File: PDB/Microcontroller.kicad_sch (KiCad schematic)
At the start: 14 parts, among them J4 Conn_01x02_Pin, U10 Thermal Resistor, U2 ESP32-DEVKIT-C, U6 TJA1050T/CM,118, U7 SparkFun: ISM330DHCX, MMC5983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, U8 SDIO Card Breakout Board, U9 AM2302

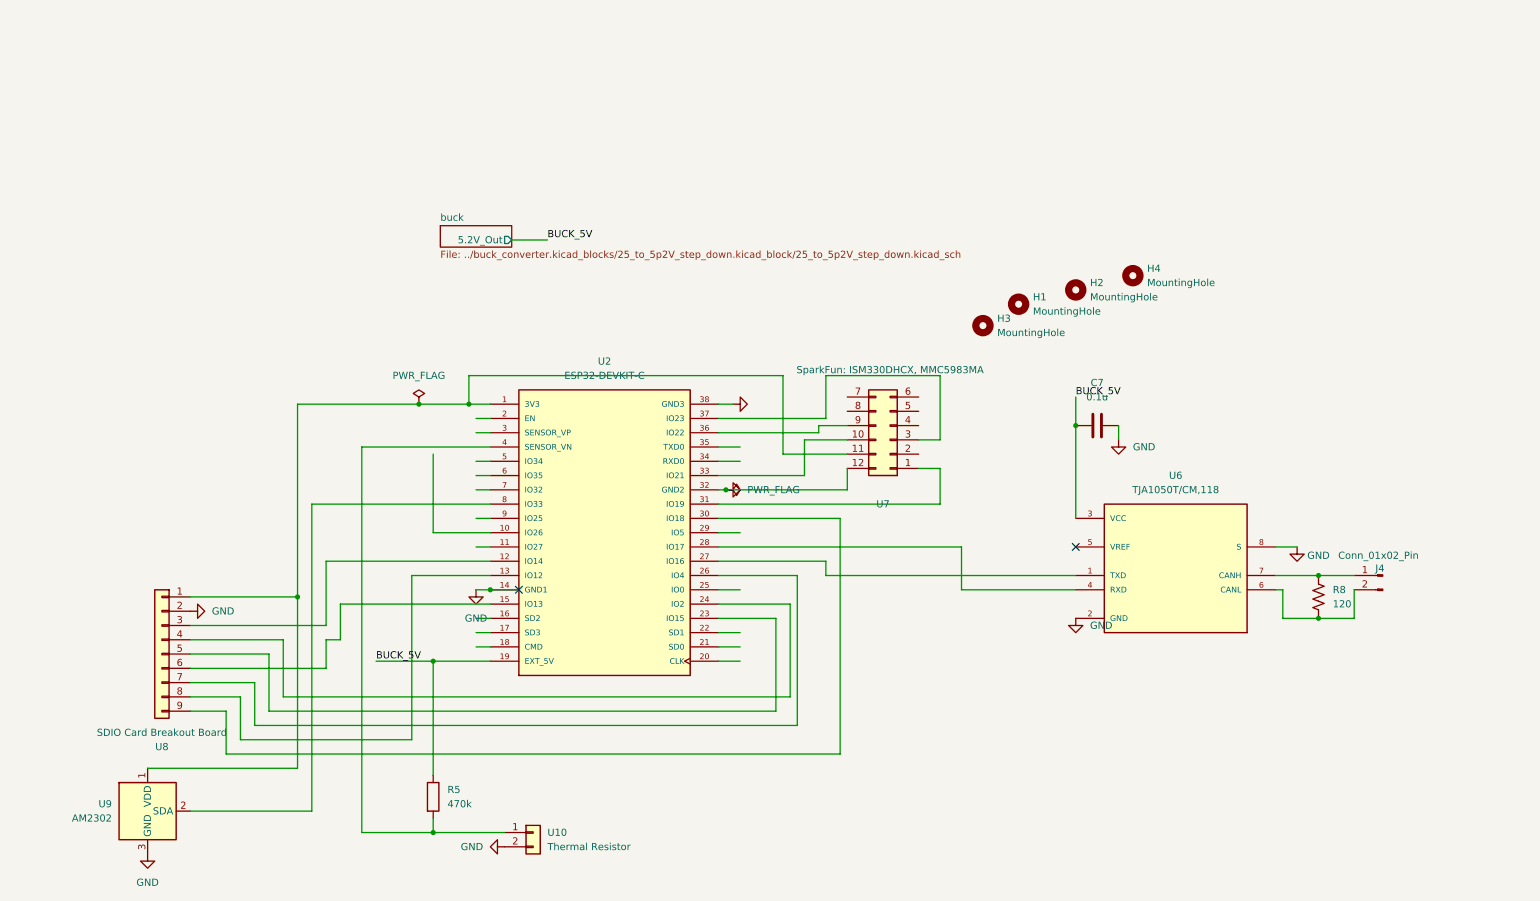
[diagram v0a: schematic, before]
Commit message: PDB_Schematic mostly updated
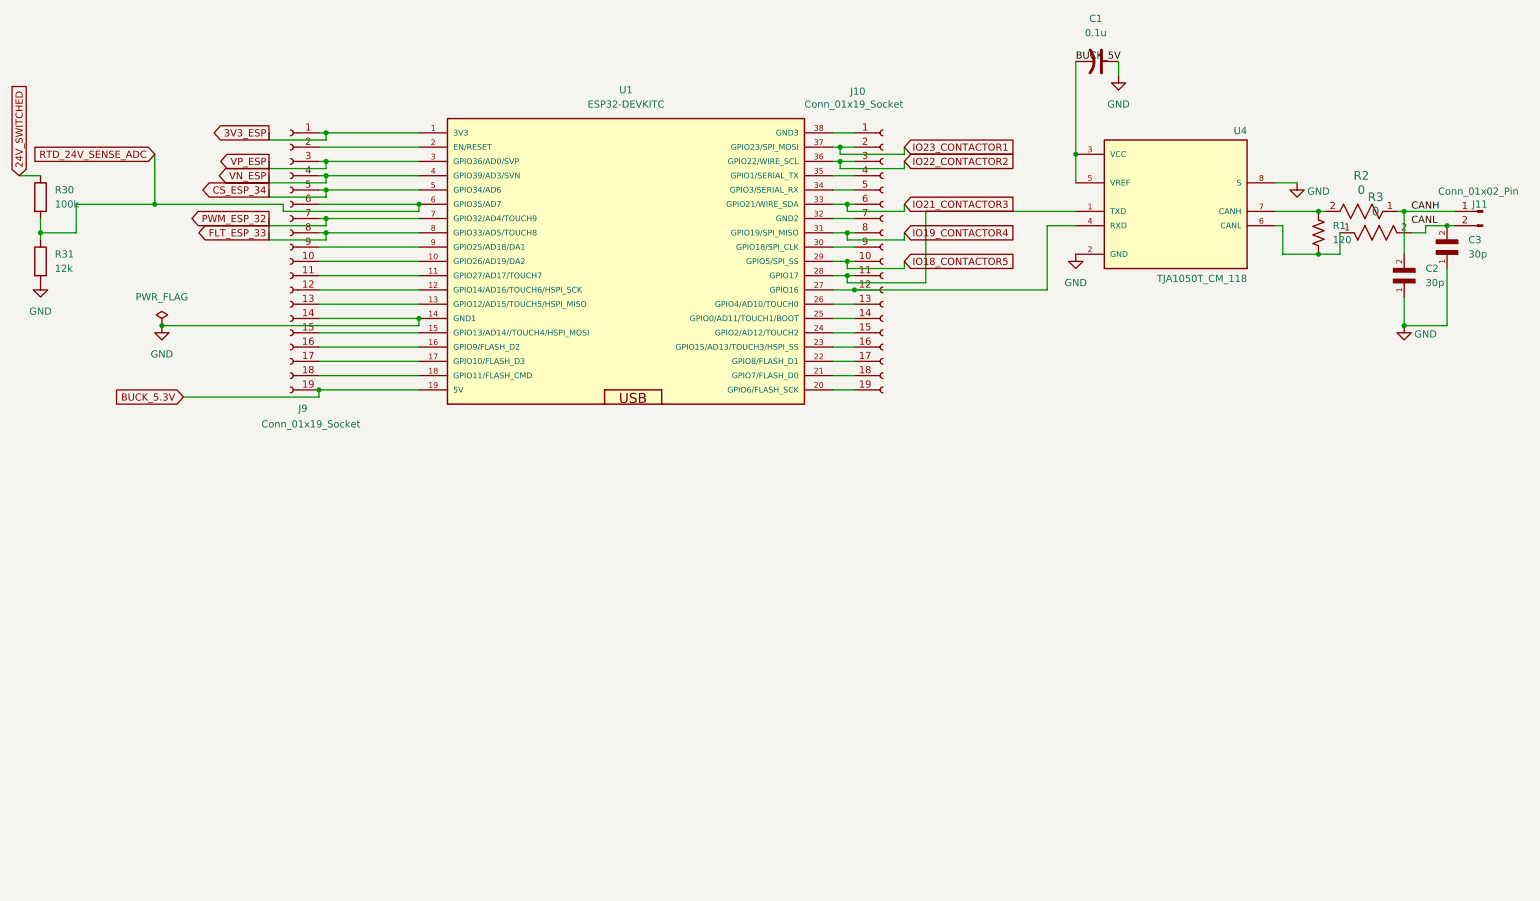
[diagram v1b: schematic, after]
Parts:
- removed H1, H2, H3, H4: MountingHole, MountingHole:MountingHole_3.2mm_M3, symbol Mechanical:MountingHole
- removed R5: 470k, Resistor_SMD:R_0805_2012Metric, symbol Device:R
- removed U10: Thermal Resistor, PROVE-footprints:TE_1877285-2, symbol Connector_Generic:Conn_01x02
- removed U7: SparkFun: ISM330DHCX, MMC5983MA, PROVE-footprints:SparkFun 9DoF IMU Breakout - ISM330DHCX, MMC5983MA (Qwiic), symbol Connector_Generic:Conn_02x06_Counter_Clockwise
- removed U8: SDIO Card Breakout Board, PROVE-footprints:Adafruit SDIO card breakout, symbol Connector_Generic:Conn_01x09
- removed U9: AM2302, Sensor:ASAIR_AM2302_P2.54mm_Vertical, symbol Sensor:AM2302
- added C2, C3: 30p, VJ1206A300JXAAT:CAPC3216X170N, symbol VJ1206A300JXAAT:VJ1206A300JXAAT
- added J10, J9: Conn_01x19_Socket, symbol Connector:Conn_01x19_Socket
- added R2, R3: 0, STA_RMCF1206_STP, symbol 2026-07-01_04-07-54:RMCF1206ZT0R00
- added R30: 100k, Resistor_SMD:R_1206_3216Metric_Pad1.30x1.75mm_HandSolder, symbol Device:R
- added R31: 12k, Resistor_SMD:R_1206_3216Metric_Pad1.30x1.75mm_HandSolder, symbol Device:R
- C1: renamed from C7; symbol PROVE:1206B104K500CT -> Device:C_US
- J11: renamed from J4; footprint PROVE-footprints:TE_1877285-2 -> (none)
- R1: renamed from R8; symbol PROVE:RMCF1206JT120R -> Device:R_US
- U1: renamed from U2; value ESP32-DEVKIT-C -> ESP32-DEVKITC; footprint PROVE-footprints:MODULE_ESP32-DEVKITC -> ESP32-DEVKITC:ESP32-DEVKITC; symbol PROVE:ESP32-DEVKIT-C -> ESP32-DEVKIT-C:ESP32-DEVKITC; Availability Not in stock -> In Stock; Check_prices https://www.snapeda.com/parts/ESP32-DEVKITC/Espressif+Syste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 -> https://www.snapeda.com/parts/ESP32-DevKitC/Espressif+Syste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; Description_1 ESP32-WROOM-32UE series Transceiver; 802.11 b/g/n (Wi-Fi, W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 -> - ESP-WROOM-32 Transceiver; 802.11 b/g/n (Wi-Fi, WiFi, WLAN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; MP ESP32-DEVKITC -> ESP32-DevKitC; Purchase-URL (none) -> https://www.snapeda.com/api/url_track_click_mouser/?unipart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; SnapEDA_Link https://www.snapeda.com/parts/ESP32-DEVKITC/Espressif+Syste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 -> https://www.snapeda.com/parts/ESP32-DevKitC/Espressif+Syste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
- U4: renamed from U6; value TJA1050T/CM,118 -> TJA1050T_CM_118; footprint Package_SO:SOIC-8_3.9x4.9mm_P1.27mm -> TJA1050T_CM_118:SOIC127P600X175-8N; symbol PROVE:TJA1050T/CM,118 -> TJA1050T_CM_118:TJA1050T_CM_118
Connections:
- net BUCK_5V: now also U4.5 (VREF); no longer U1.19 (EXT_5V)
- net GND: now also C2.1, C3.1, J9.14 (Pin_14), R31.2; no longer U1.32 (GND2), U1.38 (GND3)
- net 3V3_ESP: now reaches U1.1 (3V3)
- net 3V3_ESP: now also J9.1 (Pin_1)
- net at U1.12 (GPIO14/AD16/TOUCH6/HSPI_SCK): now also J9.12 (Pin_12)
- net at U1.24 (GPIO2/AD12/TOUCH2): now also J10.15 (Pin_15)
- net at U1.23 (GPIO15/AD13/TOUCH3/HSPI_SS): now also J10.16 (Pin_16)
- net at U1.15 (GPIO13/AD14//TOUCH4/HSPI_MOSI): now also J9.15 (Pin_15)
- net at U1.26 (GPIO4/AD10/TOUCH0): now also J10.13 (Pin_13)
- net at U1.13 (GPIO12/AD15/TOUCH5/HSPI_MISO): now also J9.13 (Pin_13)
- net at U1.30 (GPIO18/SPI_CLK): now also J10.9 (Pin_9)
- net VN_ESP: now reaches U1.4 (GPIO39/AD3/SVN)
- net VN_ESP: now also J9.4 (Pin_4)
- net at R1.1, U4.7 (CANH): now also R2.2; no longer J11.1 (Pin_1)
- net at R1.2, U4.6 (CANL): now also R3.1; no longer J11.2 (Pin_2)
- net IO19_CONTACTOR4: now reaches U1.31 (GPIO19/SPI_MISO)
- net IO19_CONTACTOR4: now also J10.8 (Pin_8)
- net IO21_CONTACTOR3: now reaches U1.33 (GPIO21/WIRE_SDA)
- net IO21_CONTACTOR3: now also J10.6 (Pin_6)
- net IO23_CONTACTOR1: now reaches U1.37 (GPIO23/SPI_MOSI)
- net IO23_CONTACTOR1: now also J10.2 (Pin_2)
- net IO22_CONTACTOR2: now reaches U1.36 (GPIO22/WIRE_SCL)
- net IO22_CONTACTOR2: now also J10.3 (Pin_3)
- net FLT_ESP_33: now reaches U1.8 (GPIO33/AD5/TOUCH8)
- net FLT_ESP_33: now also J9.8 (Pin_8)
- net at U1.10 (GPIO26/AD19/DA2): now also J9.10 (Pin_10)
- net at U1.11 (GPIO27/AD17/TOUCH7): now also J9.11 (Pin_11)
- net at U1.16 (GPIO9/FLASH_D2): now also J9.16 (Pin_16)
- net at U1.17 (GPIO10/FLASH_D3): now also J9.17 (Pin_17)
- net at U1.18 (GPIO11/FLASH_CMD): now also J9.18 (Pin_18)
- net at U1.2 (EN/RESET): now also J9.2 (Pin_2)
- net at U1.20 (GPIO6/FLASH_SCK): now also J10.19 (Pin_19)
- net at U1.21 (GPIO7/FLASH_D0): now also J10.18 (Pin_18)
- net at U1.22 (GPIO8/FLASH_D1): now also J10.17 (Pin_17)
- net at U1.25 (GPIO0/AD11/TOUCH1/BOOT): now also J10.14 (Pin_14)
- net at U4.1 (TXD): now also U1.28 (GPIO17), J10.11 (Pin_11); no longer U1.27 (IO16)
- net at U4.4 (RXD): now also U1.27 (GPIO16), J10.12 (Pin_12); no longer U1.28 (IO17)
- net IO18_CONTACTOR5: now reaches U1.29 (GPIO5/SPI_SS)
- net IO18_CONTACTOR5: now also J10.10 (Pin_10)
- net VP_ESP: now reaches U1.3 (GPIO36/AD0/SVP)
- net VP_ESP: now also J9.3 (Pin_3)
- net at U1.34 (GPIO3/SERIAL_RX): now also J10.5 (Pin_5)
- net at U1.35 (GPIO1/SERIAL_TX): now also J10.4 (Pin_4)
- net CS_ESP_34: now reaches U1.5 (GPIO34/AD6)
- net CS_ESP_34: now also J9.5 (Pin_5)
- net RTD_24V_SENSE_ADC: now reaches U1.6 (GPIO35/AD7)
- net RTD_24V_SENSE_ADC: now also J9.6 (Pin_6), R30.2, R31.1
- net PWM_ESP_32: now reaches U1.7 (GPIO32/AD4/TOUCH9)
- net PWM_ESP_32: now also J9.7 (Pin_7)
- net at U1.9 (GPIO25/AD18/DA1): now also J9.9 (Pin_9)
- new net: C3.2, J11.2 (Pin_2), R3.2
- new net: J10.1 (Pin_1), U1.38 (GND3)
- new net: J10.7 (Pin_7), U1.32 (GND2)
- new net 24V_SWITCHED: R30.1
- new net BUCK_5.3V: J9.19 (Pin_19), U1.19 (5V)
- new net CANH: C2.2, J11.1 (Pin_1), R2.1
- no-connect marks 2 -> 0
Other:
- removed sheet buck
- company: PROVE Lab, Julia Kohrt -> (none)
- title: IMU Board -> (none)
- moved on the sheet: C1, J11, R1, U4
